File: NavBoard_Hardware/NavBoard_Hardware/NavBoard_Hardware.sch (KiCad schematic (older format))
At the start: 61 parts, among them U1 OKI-5V, U2 ICM-20948, U3 BNO055, U4 OKI-3V3, U5 NEO-M8P-2, U6 Raspberry_Pi

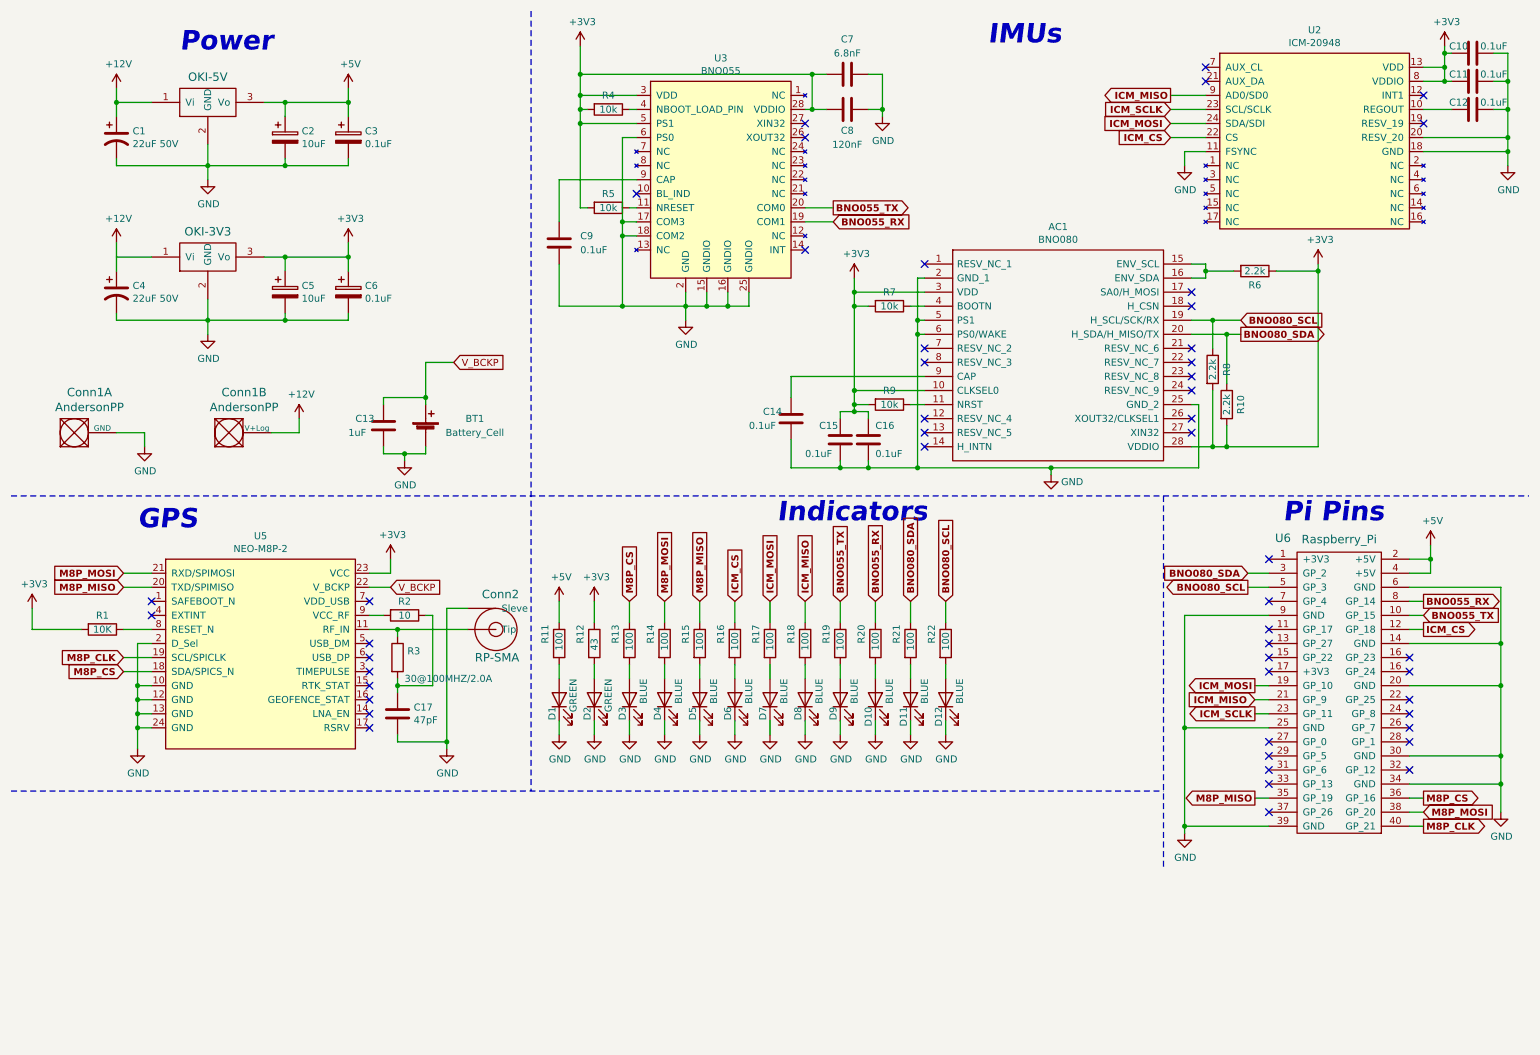
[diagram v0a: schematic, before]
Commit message: Deleted old components
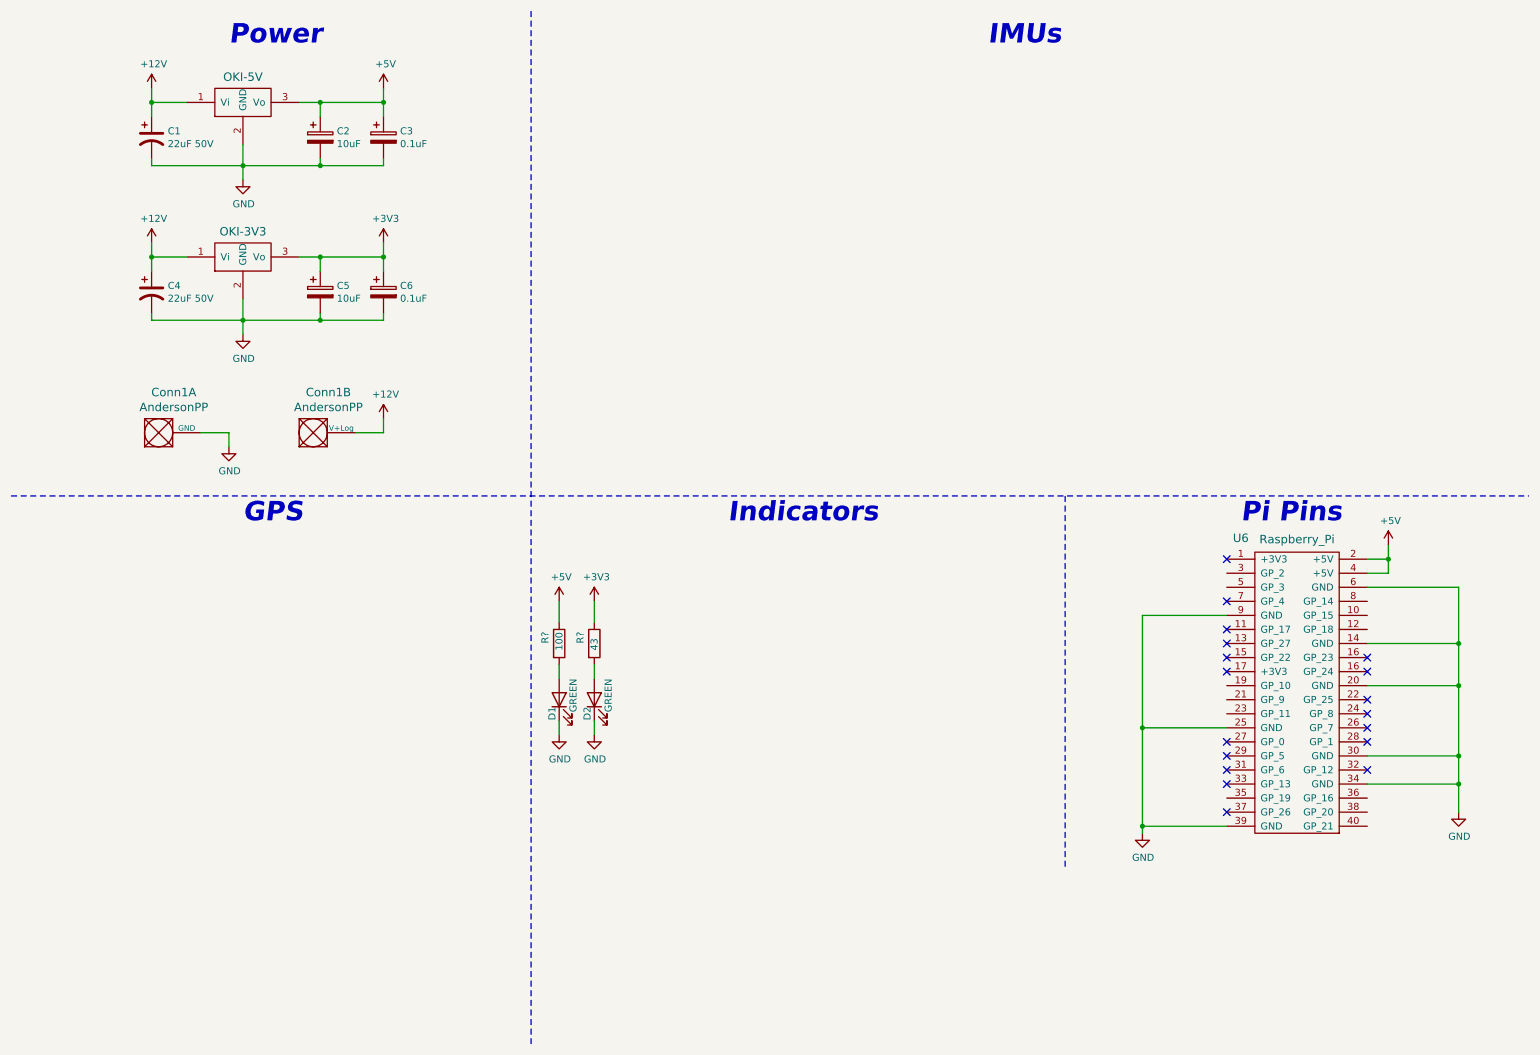
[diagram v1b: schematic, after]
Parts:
- removed AC1: BNO080, BNO080:BNO080, symbol NavBoard_Hardware-rescue:BNO080-BNO080
- removed BT1: Battery_Cell, Battery:BatteryHolder_Keystone_3008_1x2450, symbol Device:Battery_Cell
- removed C10, C11, C12, C14, C15, C16, C9: 0.1uF, Capacitor_SMD:C_0603_1608Metric_Pad1.08x0.95mm_HandSolder, symbol Device:C
- removed C13: 1uF, Capacitor_SMD:C_0603_1608Metric_Pad1.08x0.95mm_HandSolder, symbol Device:C
- removed C17: 47pF, Capacitor_SMD:C_0603_1608Metric_Pad1.08x0.95mm_HandSolder, symbol Device:C
- removed C7: 6.8nF, Capacitor_SMD:C_0603_1608Metric_Pad1.08x0.95mm_HandSolder, symbol Device:C
- removed C8: 120nF, Capacitor_SMD:C_0603_1608Metric_Pad1.08x0.95mm_HandSolder, symbol Device:C
- removed Conn2: RP-SMA, MRDT_Connectors:RP-SMA_Jack_Tru-Hole_Right-Angle, symbol NavBoard_Hardware-rescue:RP-SMA-MRDT_Connectors
- removed D10, D11, D12, D3, D4, D5, D6, D7, D8, D9: BLUE, LED_SMD:LED_0603_1608Metric_Pad1.05x0.95mm_HandSolder, symbol Device:LED
- removed R1: 10K, Resistor_SMD:R_0603_1608Metric_Pad0.98x0.95mm_HandSolder, symbol Device:R
- removed R10, R6, R8: 2.2k, Resistor_SMD:R_0603_1608Metric_Pad0.98x0.95mm_HandSolder, symbol Device:R
- removed R13, R14, R15, R16, R17, R18, R19, R20, R21, R22: 100, Resistor_SMD:R_0603_1608Metric_Pad0.98x0.95mm_HandSolder, symbol Device:R
- removed R2: 10, Resistor_SMD:R_0603_1608Metric_Pad0.98x0.95mm_HandSolder, symbol Device:R
- removed R3: 30@100MHZ/2.0A, Resistor_SMD:R_0603_1608Metric_Pad0.98x0.95mm_HandSolder, symbol Device:R
- removed R4, R5, R7, R9: 10k, Resistor_SMD:R_0603_1608Metric_Pad0.98x0.95mm_HandSolder, symbol Device:R
- removed U2: ICM-20948, MRDT_ICs:ICM_20948, symbol NavBoard_Hardware-rescue:ICM-20948-MRDT_ICs
- removed U3: BNO055, MRDT_ICs:BNO055, symbol NavBoard_Hardware-rescue:BNO055-MRDT_ICs
- removed U5: NEO-M8P-2, MRDT_ICs:MODULE_NEO-M8P-2, symbol NavBoard_Hardware-rescue:NEO-M8P-2-MRDT_ICs
- renumbered R11 to R?, R12 to R?
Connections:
- net BNO055_RX: no longer names the net of U6.8 (GP_14)
- net BNO055_TX: no longer names the net of U6.10 (GP_15)
- net BNO080_SCL: no longer names the net of U6.5 (GP_3)
- net BNO080_SDA: no longer names the net of U6.3 (GP_2)
- net ICM_CS: no longer names the net of U6.12 (GP_18)
- net ICM_MISO: no longer names the net of U6.21 (GP_9)
- net ICM_MOSI: no longer names the net of U6.19 (GP_10)
- net ICM_SCLK: no longer names the net of U6.23 (GP_11)
- net M8P_CLK: no longer names the net of U6.40 (GP_21)
- net M8P_CS: no longer names the net of U6.36 (GP_16)
- net M8P_MISO: no longer names the net of U6.35 (GP_19)
- net M8P_MOSI: no longer names the net of U6.38 (GP_20)
- no-connect marks 50 -> 18
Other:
- moved on the sheet: C1, C2, C3, C4, C5, C6, Conn1A, Conn1B, U6
